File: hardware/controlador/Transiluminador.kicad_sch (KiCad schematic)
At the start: 85 parts, among them J1 Conn_01x03_Pin, J10 USB_B_Micro, J11 V_in, J12 V_DD, J13 GND, J14 5V, J15 3.3V, J16 VDL_3V3, J17 VS_3V3, J2 Conn_01x03_Pin, J3 HDR-2x1, J4 Conn_01x03_Pin, J5 Conn_01x03_Pin, J6 Conn_01x05_Pin, J7 HDR-3x1, J8 ST77XX, J9 HDR-3x1, Q1 Q_PMOS_GSD, Q4 Q_Dual_NPN_NPN_BRT_E1B1C2E2B2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, SW2 SW_DIP_x02, SW3 SW_DIP_x02, U10 ESP32-WROOM-32D, U4 MT3608, U6 AP2112K-3.3, U7 AP2112K-3.3, U8 AP2112K-3.3, U9 CH340C

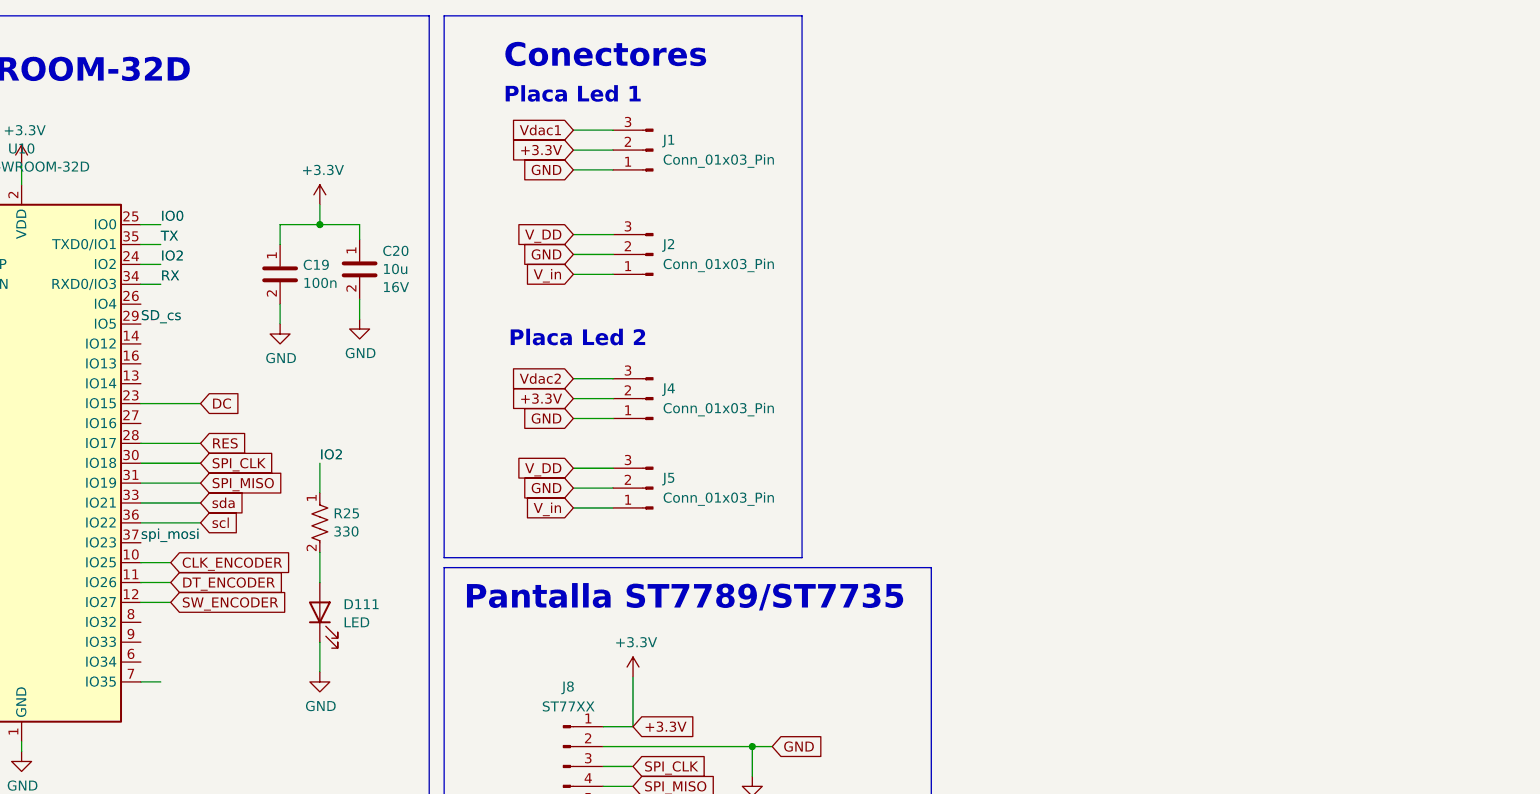
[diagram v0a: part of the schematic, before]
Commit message: pcb
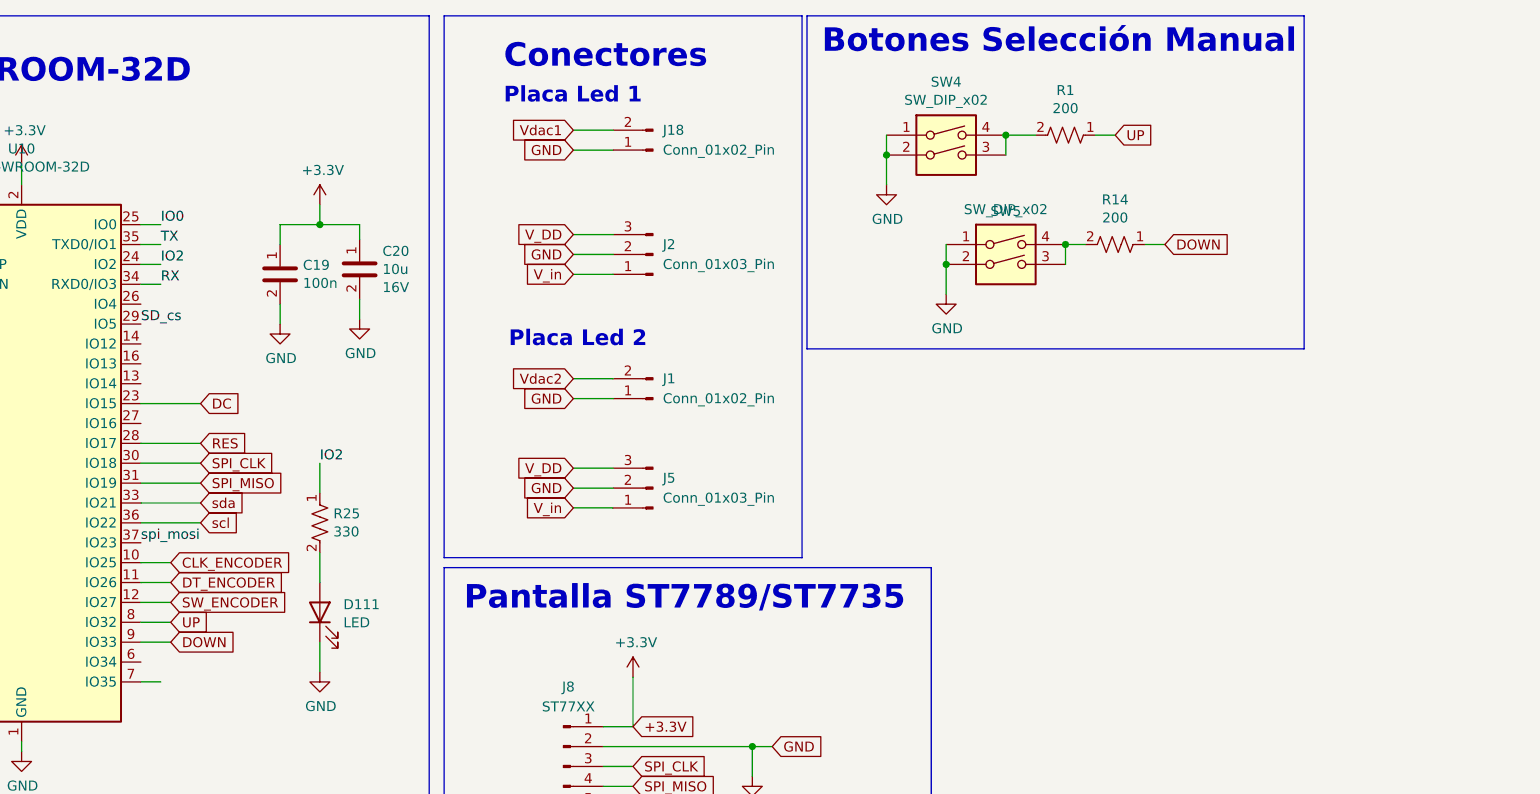
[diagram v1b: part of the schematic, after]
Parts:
- removed J1, J4: Conn_01x03_Pin, Connector_JST:JST_XH_B3B-XH-A_1x03_P2.50mm_Vertical, symbol Connector:Conn_01x03_Pin
- added J1, J18: Conn_01x02_Pin, Connector_JST:JST_XH_B2B-XH-A_1x02_P2.50mm_Vertical, symbol Connector:Conn_01x02_Pin
- added R1, R14: 200, Resistor_SMD:R_0603_1608Metric, symbol IoWLabs:RES
- added SW4, SW5: SW_DIP_x02, IoWLabs:SMD_SWITCH, symbol Switch:SW_DIP_x02
- J11, J12, J13, J14, J15, J16, J17: footprint (none) -> TestPoint:TestPoint_Loop_D2.50mm_Drill1.0mm_LowProfile
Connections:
- net GND: now also J1.1 (Pin_1), J18.1 (Pin_1), SW4.1, SW4.2, SW5.1, SW5.2
- net Vdac1: now also J18.2 (Pin_2)
- net Vdac2: now also J1.2 (Pin_2)
- net UP: now reaches U10.8 (IO32)
- net UP: now also R1.1
- net DOWN: now reaches U10.9 (IO33)
- net DOWN: now also R14.1
- new net: R1.2, SW4.3, SW4.4
- new net: R14.2, SW5.3, SW5.4
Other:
- note added: "Botones Selección Manual"
